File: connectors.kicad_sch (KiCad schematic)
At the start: 11 parts, among them J1 Conn_01x05, J2 AudioJack3, J3 USB_A, J4 Conn_01x03

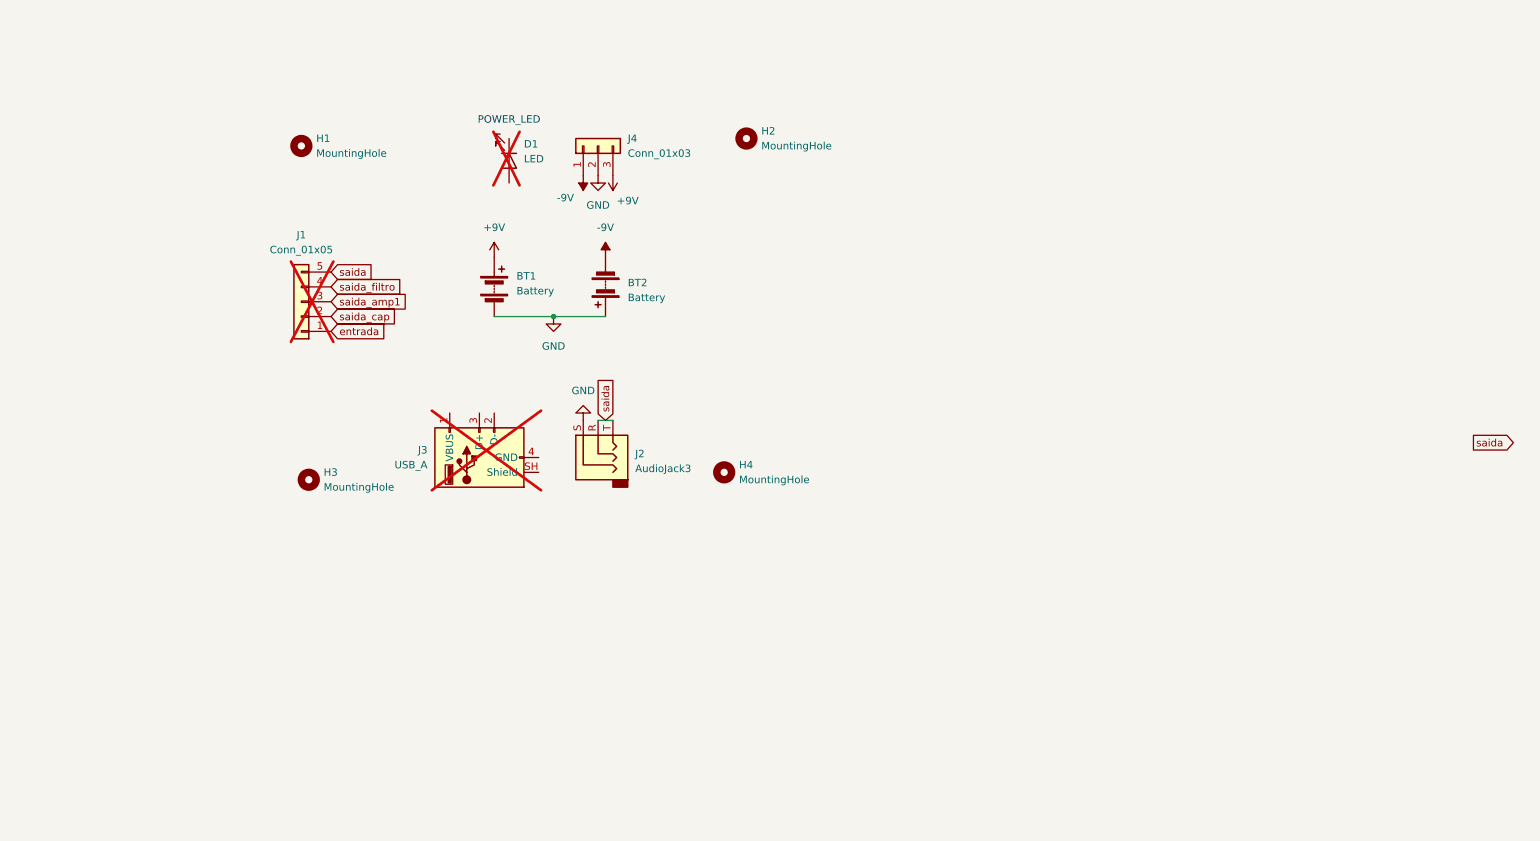
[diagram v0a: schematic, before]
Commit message: Done
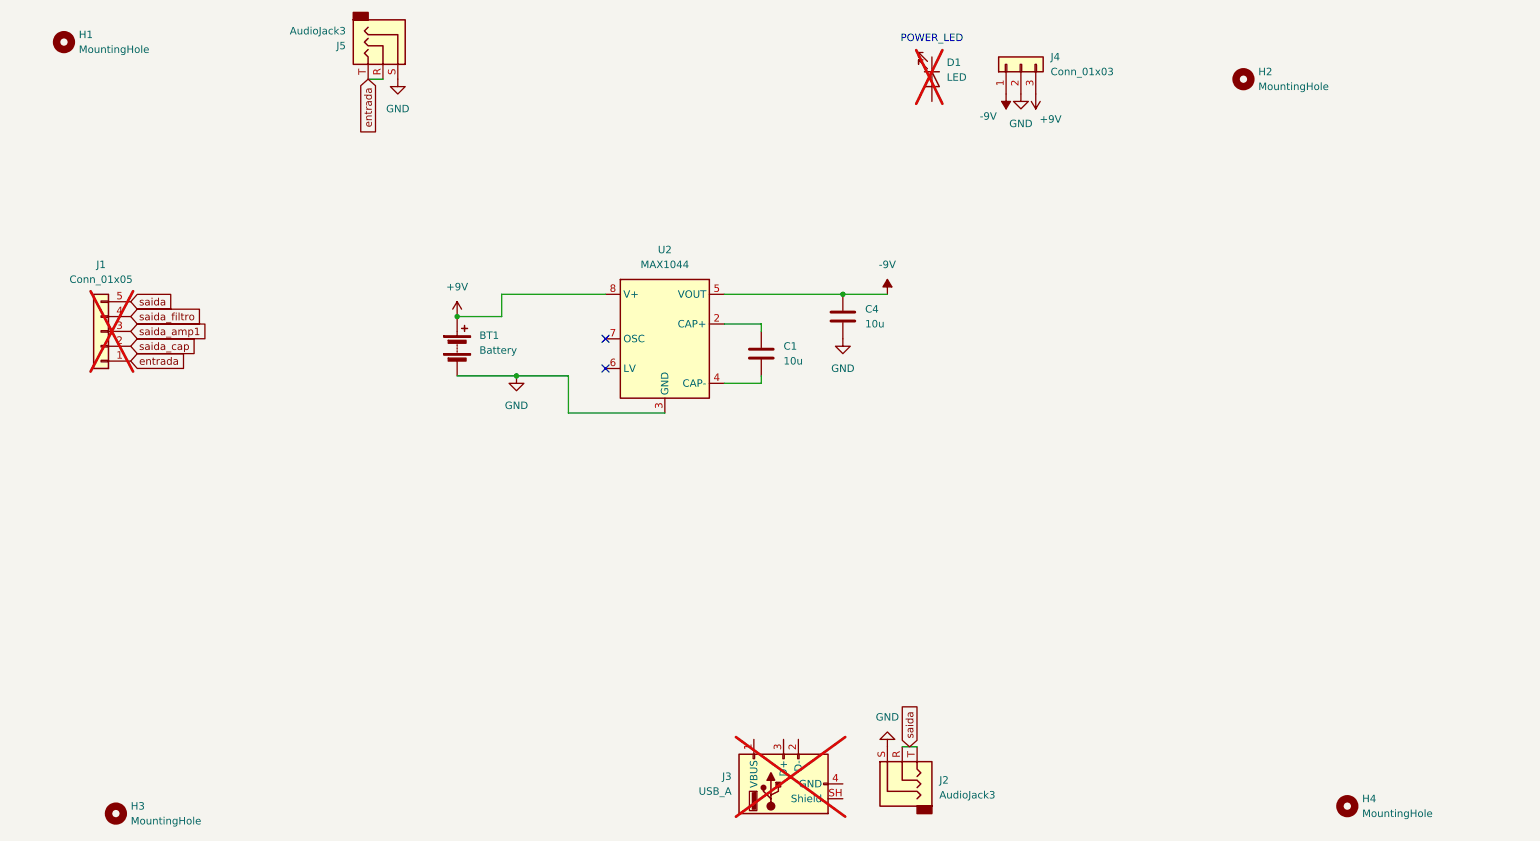
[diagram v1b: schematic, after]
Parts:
- removed BT2: Battery, Beserrovsky:BatteryHolder_Eagle_12BH611-GR, symbol Device:Battery
- added C1, C4: 10u, Capacitor_SMD:C_1206_3216Metric, symbol Device:C
- added J5: AudioJack3, Connector_Audio:Jack_3.5mm_CUI_SJ1-3525N_Horizontal, symbol Connector_Audio:AudioJack3
- added U2: MAX1044, Package_SO:SOIC-8_3.9x4.9mm_P1.27mm, symbol Regulator_SwitchedCapacitor:MAX1044
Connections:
- net +9V: now also U2.8 (V+)
- net -9V: now also C4.1, U2.5 (VOUT)
- net GND: now also C4.2, J5.S, U2.3 (GND)
- net entrada: now also J5.R, J5.T
- new net: C1.1, U2.2 (CAP+)
- new net: C1.2, U2.4 (CAP-)
- no-connect marks 0 -> 2
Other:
- moved on the sheet: BT1, D1, H1, H2, H3, H4, J1, J2, J3, J4

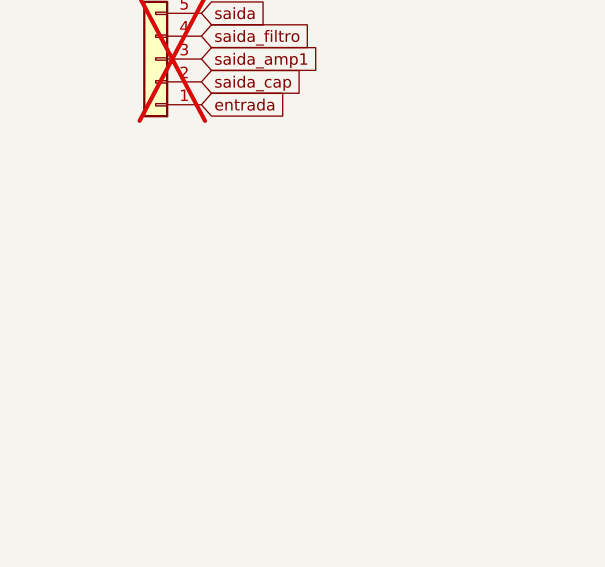
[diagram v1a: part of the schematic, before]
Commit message: kinda broken state
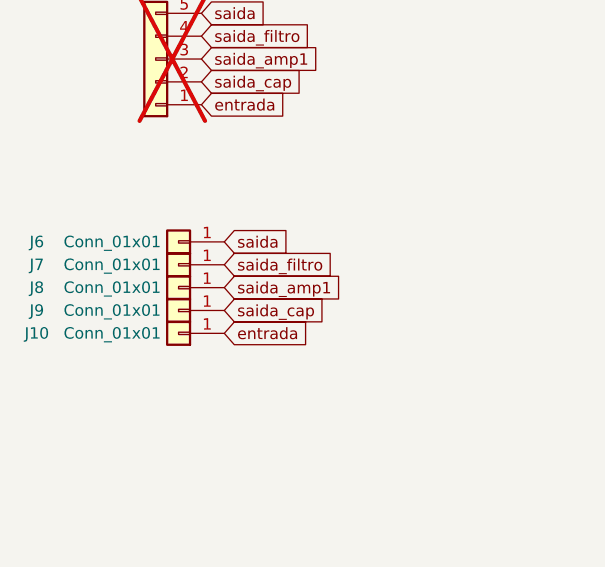
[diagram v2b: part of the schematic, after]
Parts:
- added J10, J6, J7, J8, J9: Conn_01x01, TestPoint:TestPoint_Pad_1.5x1.5mm, symbol Connector_Generic:Conn_01x01
- J3: FootPrintAlternativo (none) -> USB_A_Molex_67643_Horizontal
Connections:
- net entrada: now also J10.1 (Pin_1)
- net saida: now also J6.1 (Pin_1)
- net saida_amp1: now also J8.1 (Pin_1)
- net saida_cap: now also J9.1 (Pin_1)
- net saida_filtro: now also J7.1 (Pin_1)
